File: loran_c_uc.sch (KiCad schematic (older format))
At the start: 39 parts, among them U701 STM32F407VG, X701 32.768KHz

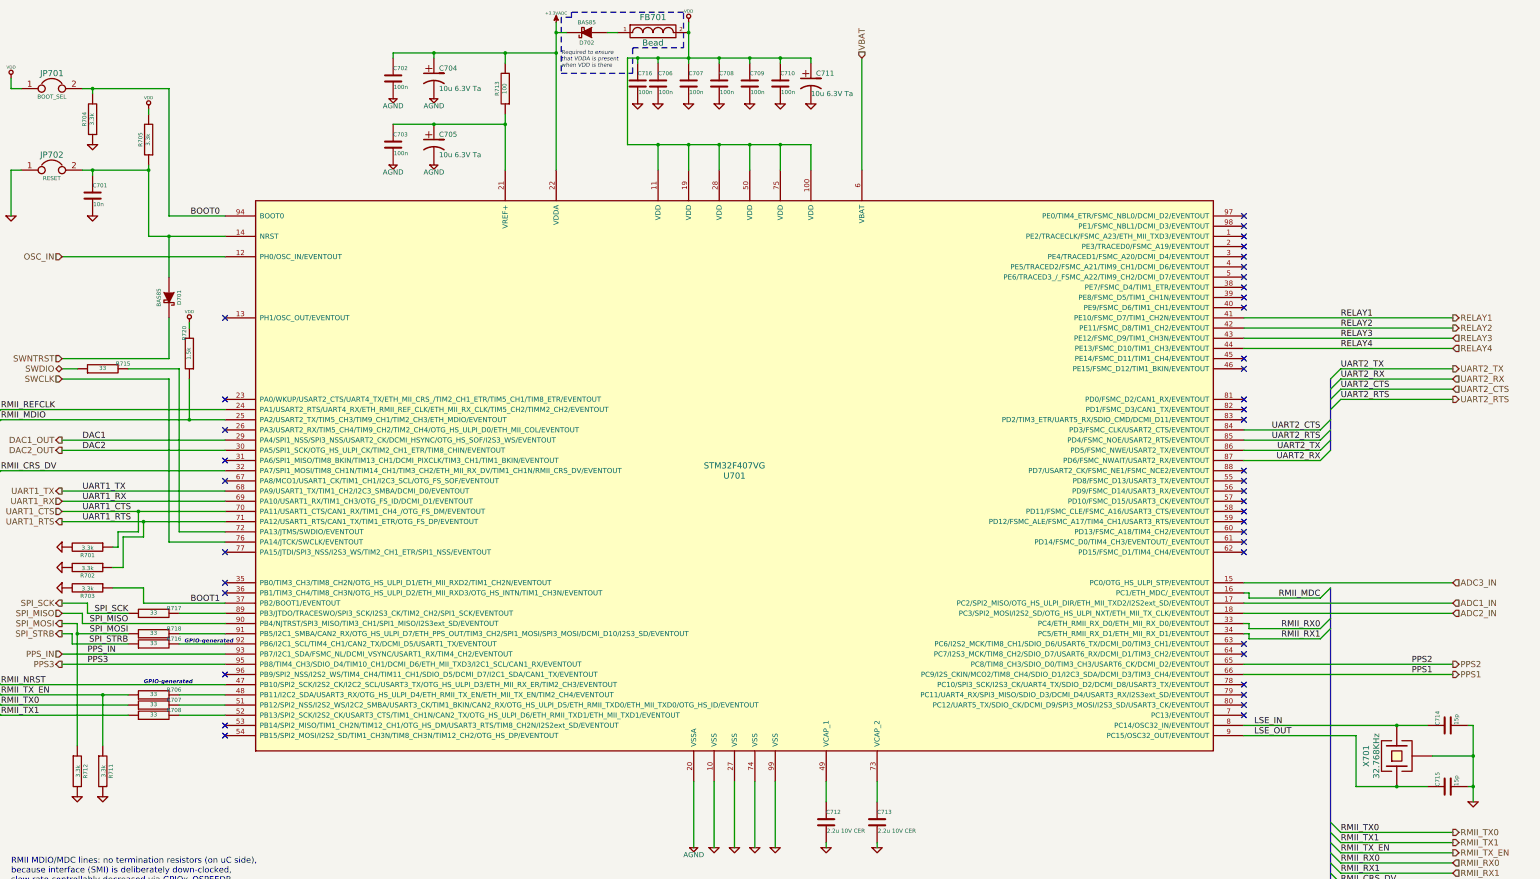
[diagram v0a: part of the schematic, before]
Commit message: Update: PCB almost finished (3D views also up-to-date)
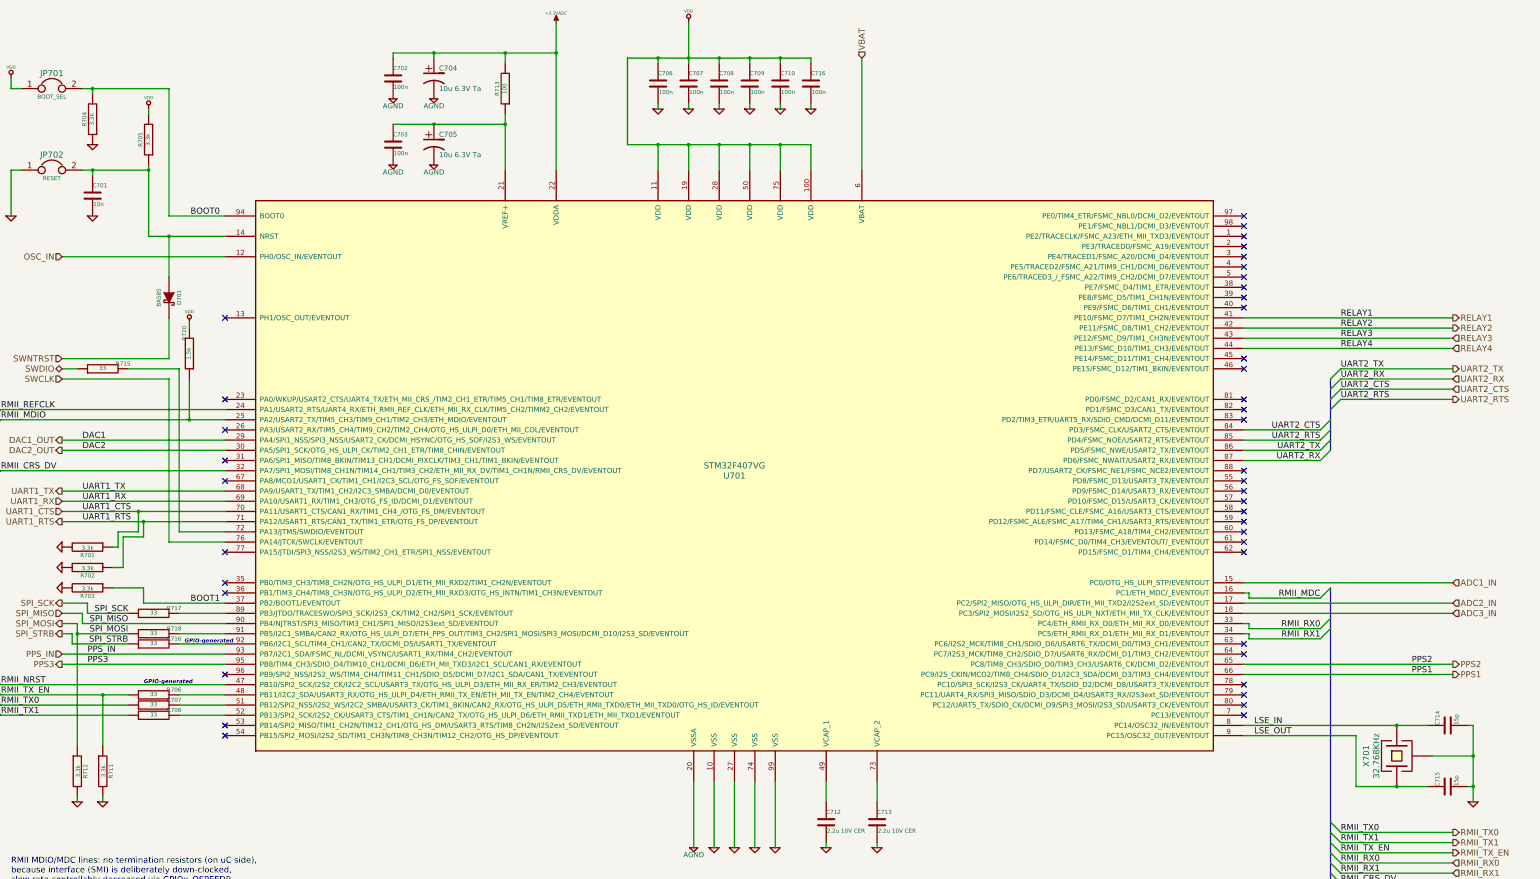
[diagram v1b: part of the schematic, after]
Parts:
- removed C711: 10u 6.3V Ta, w_smd_capacitors:c_tant_B, symbol CP1
- removed D702: BAS85, w_smd_diode:sod80c, symbol DIODESCH
- removed FB701: Bead, w_pth_resistors:RC07, symbol FILTER
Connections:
- net ADC1_IN: now also U701.15 (PC0/OTG_HS_ULPI_STP/EVENTOUT); no longer U701.17 (PC2/SPI2_MISO/OTG_HS_ULPI_DIR/ETH_MII_TXD2/I2S2ext_SD/EVENTOUT)
- net ADC2_IN: now also U701.17 (PC2/SPI2_MISO/OTG_HS_ULPI_DIR/ETH_MII_TXD2/I2S2ext_SD/EVENTOUT); no longer U701.18 (PC3/SPI2_MOSI/I2S2_SD/OTG_HS_ULPI_NXT/ETH_MII_TX_CLK/EVENTOUT)
- net ADC3_IN: now also U701.18 (PC3/SPI2_MOSI/I2S2_SD/OTG_HS_ULPI_NXT/ETH_MII_TX_CLK/EVENTOUT); no longer U701.15 (PC0/OTG_HS_ULPI_STP/EVENTOUT)
- net LSE_IN: now also X701.1; no longer X701.2
- net LSE_OUT: now also X701.2; no longer X701.1
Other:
- note removed: "Required to ensure\nthat VDDA is present\nwhen VDD is there"
- moved on the sheet: C716
